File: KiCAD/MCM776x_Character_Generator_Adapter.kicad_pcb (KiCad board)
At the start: 2 copper layers, 18.3 x 51.2 mm, 11 parts, among them J1 Conn_02x05_Odd_Even, J2 Conn_02x06_Odd_Even, U1 Conn_02x09_Counter_Clockwise, U2 27512

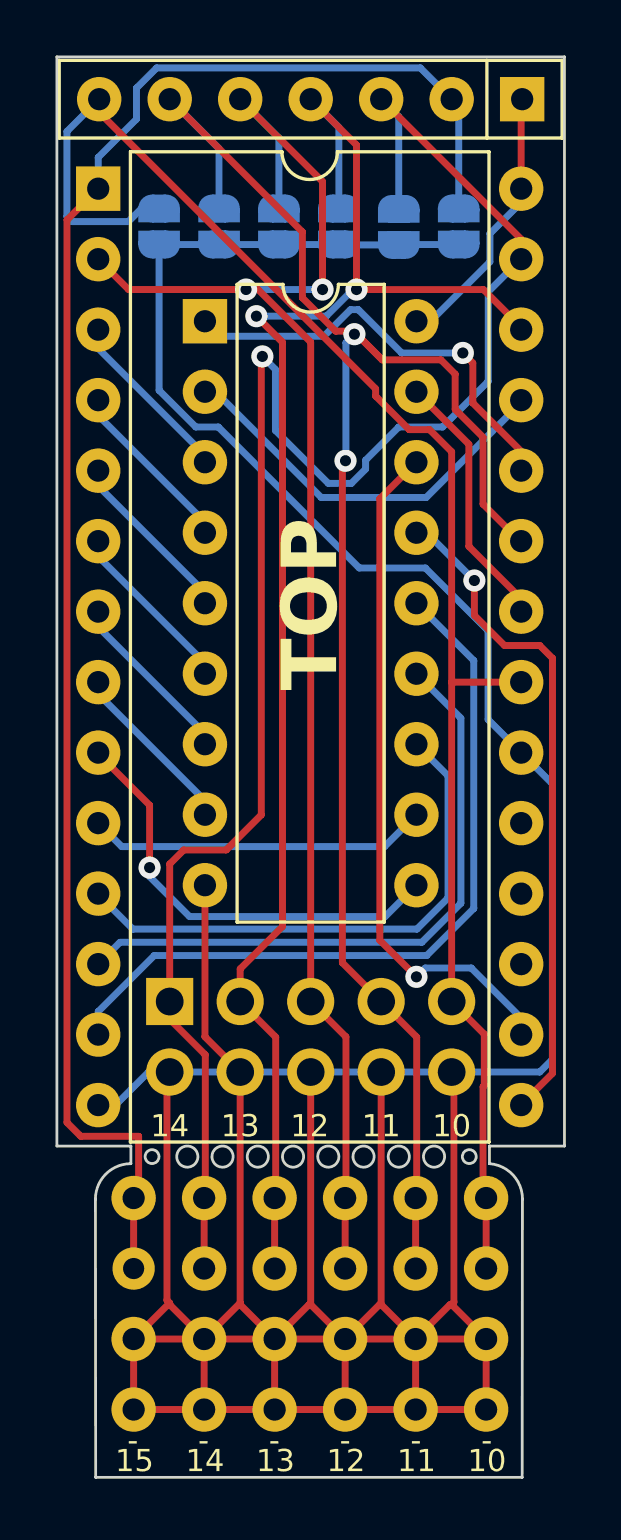
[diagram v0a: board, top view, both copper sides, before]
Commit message: Rev 1.1
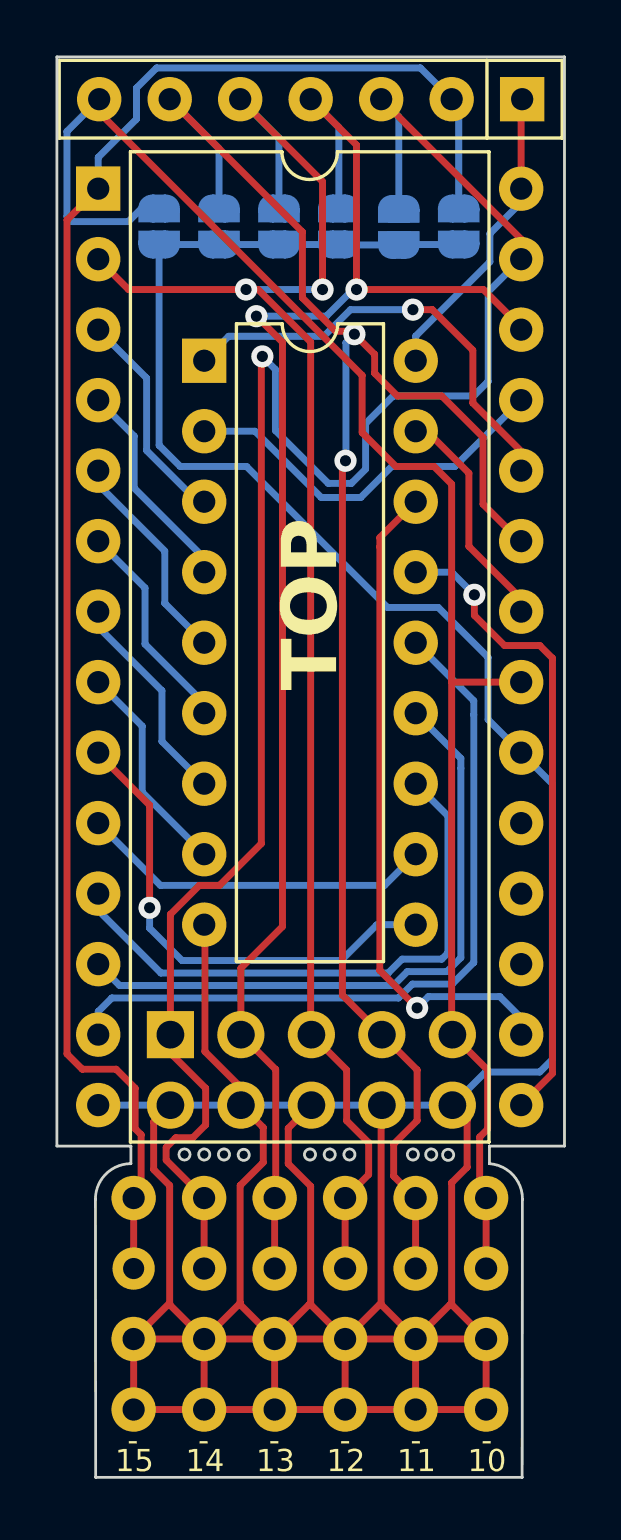
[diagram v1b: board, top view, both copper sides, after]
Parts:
- moved U1 1.42 mm to (119.0, 84.5)
- moved J1 1.19 mm to (117.8, 108.8)
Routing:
- net GND: track 172.8 -> 169.4 mm
- net /A14: track 65.7 -> 68.1 mm
- net /A1: track 15.9 -> 17.7 mm
- net /A7: track 6.37 -> 7.92 mm
- net /A2: track 6.37 -> 7.78 mm
- net /A4: track 6.37 -> 7.78 mm
- net /A6: track 6.37 -> 7.78 mm
- net /A3: track 6.37 -> 7.78 mm
- net /A5: track 6.37 -> 7.78 mm
- net /D0: track 19.6 -> 21.0 mm
- net /~{CS}: track 9.49 -> 8.31 mm
- net +5V: track 9.88 -> 11.0 mm
- net /A11: track 63.8 -> 62.8 mm
- net /D3: track 24.1 -> 23.2 mm
- net /D4: track 24.9 -> 24.2 mm
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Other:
- outline, holes or cut-outs redrawn
- board text added: "Rev 1.1"
- board text removed: "Rev 1.0"
